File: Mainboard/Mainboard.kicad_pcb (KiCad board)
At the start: 4 copper layers, 106.1 x 132 mm, 128 parts, among them IC1 REF102AU_2K5, IC4 DAC8814IBDBT, J1 5745782-6, J2 5745782-6, J3 5745782-6, J4 Conn_01x02_Pin, J5 Conn_01x02_Pin, J6 Conn_01x02_Pin, U1 Teensy4.0, U10 TL072, U11 ADG419BR, U12 ADG419BR, U2 TL072, U3 TL072, U4 TL072, U5 TL074, U6 TL074, U7 ADG419BR, U8 LTC2326CMS-16-PBF, U9 LT1469CS8-TRPBF

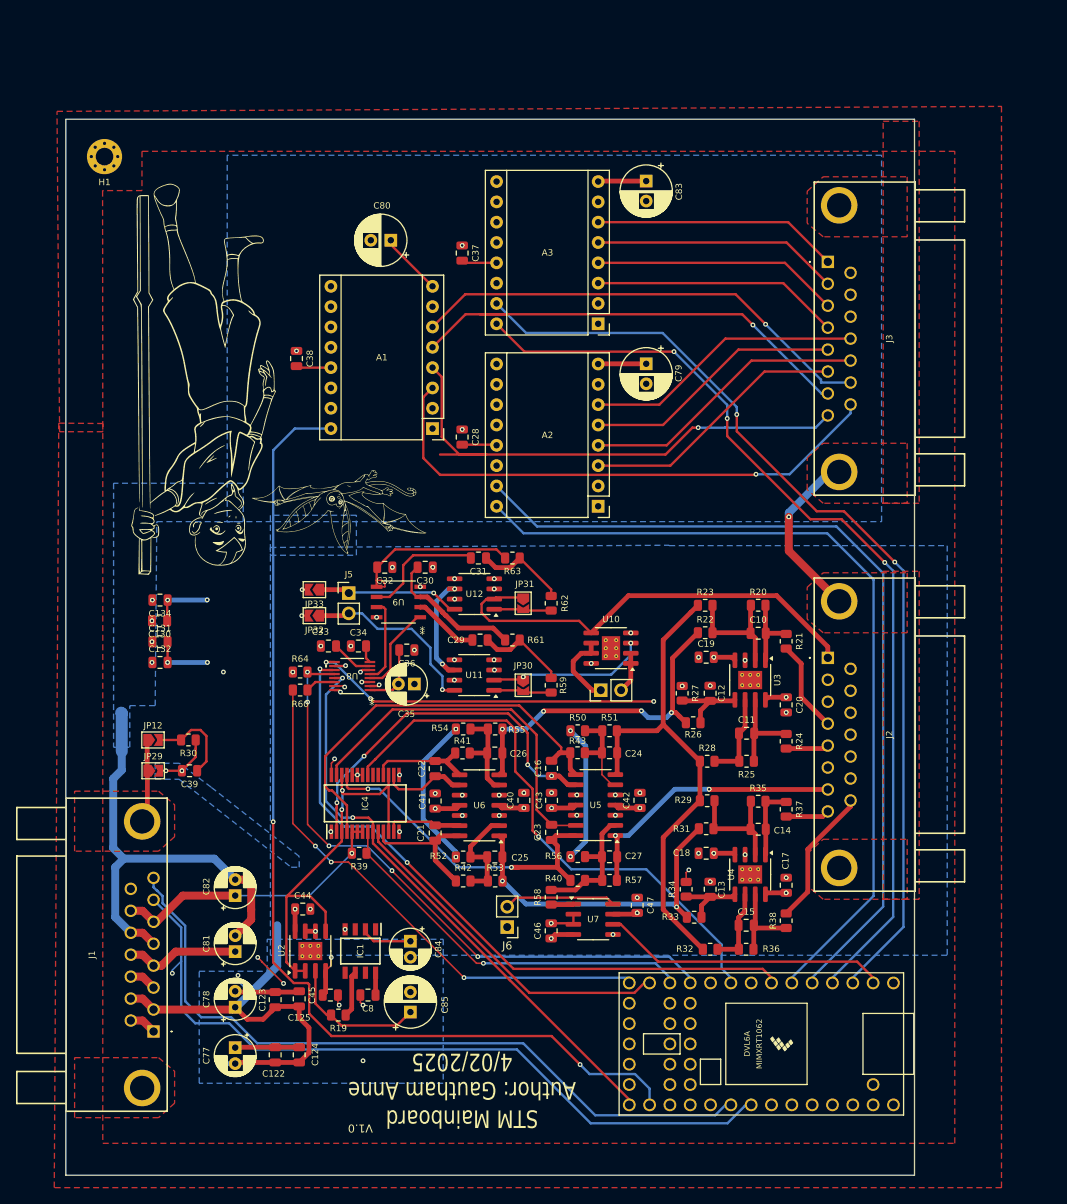
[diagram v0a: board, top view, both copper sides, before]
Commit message: caddy cad updates
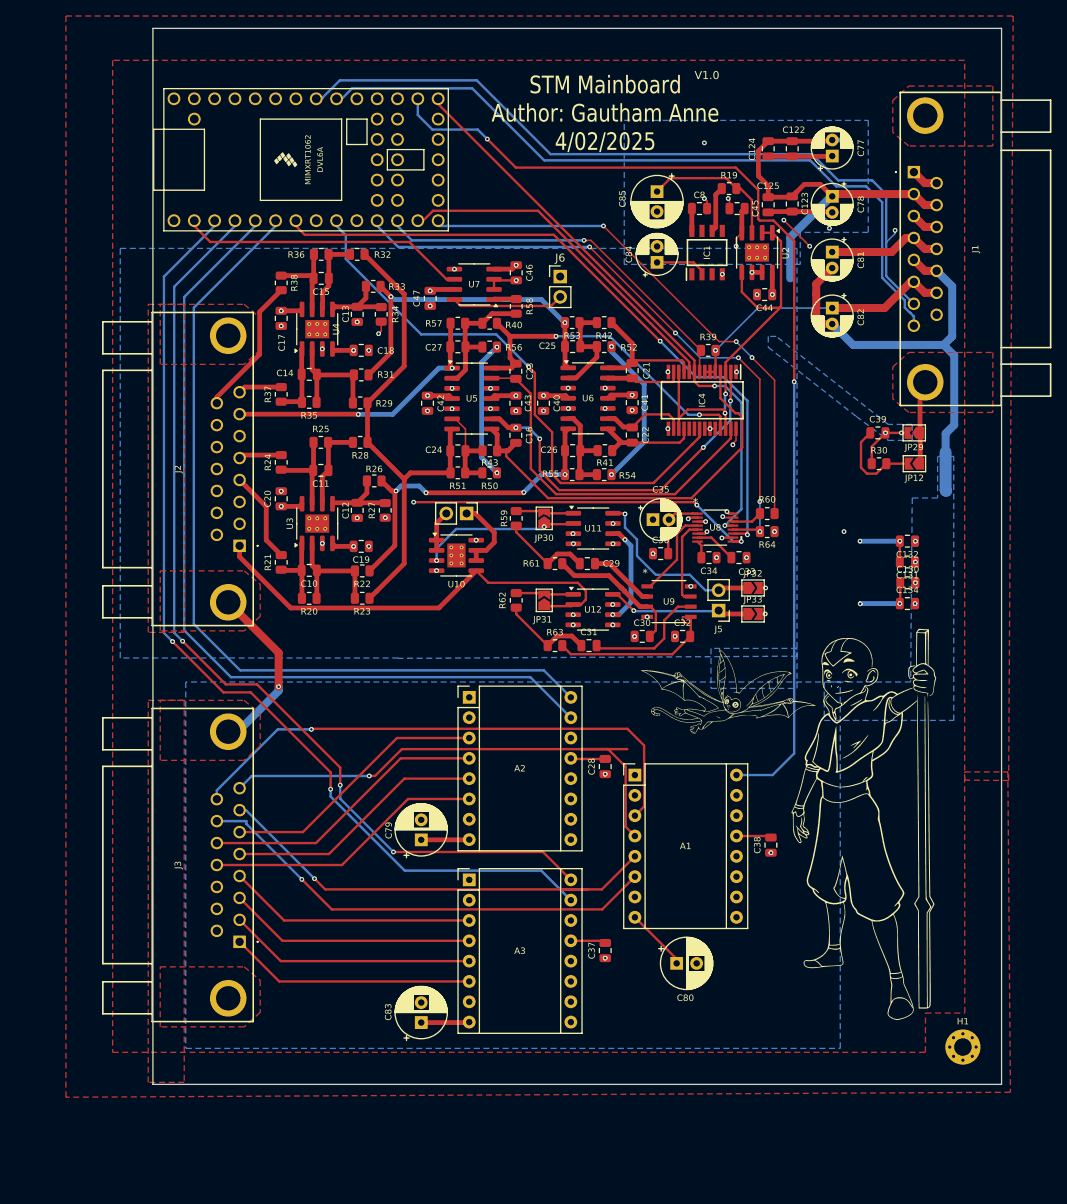
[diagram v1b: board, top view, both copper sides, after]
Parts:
- moved H1 154.6 mm to (192.4, 150.1), turned to 0 degrees
- moved J1 143.4 mm to (186.3, 40.8), turned to 90 degrees
- moved C77 134.1 mm to (176.1, 38.8), turned to 90 degrees
- moved C122 130.4 mm to (171.1, 37.9), turned to 90 degrees
- moved C124 127.5 mm to (168.1, 37.9), turned to 90 degrees
- moved C78 125.9 mm to (176.1, 43.8), turned to -90 degrees
- moved U1 124.3 mm to (110.3, 39.2), turned to 0 degrees
- moved C123 118.6 mm to (171.1, 44.8), turned to -90 degrees
- moved C125 115.3 mm to (168.1, 44.9), turned to -90 degrees
- moved C81 115.0 mm to (176.1, 50.8), turned to -90 degrees
- moved R19 114.3 mm to (163.2, 42.8), turned to 0 degrees
- moved J3 112.4 mm to (102.0, 137.0), turned to -90 degrees
- moved C45 110.7 mm to (164.2, 45.3), turned to 0 degrees
- moved C83 108.9 mm to (124.7, 147.1), turned to 90 degrees
- moved C85 107.1 mm to (154.2, 43.2), turned to -90 degrees
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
